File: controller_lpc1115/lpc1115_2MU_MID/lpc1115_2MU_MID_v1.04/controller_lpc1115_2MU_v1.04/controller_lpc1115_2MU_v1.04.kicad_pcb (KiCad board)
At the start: 2 copper layers, 32 x 58.1 mm, 66 parts, among them IC1 LPC1115, J1 Conn_App, J2 Conn_UI, J3 Conn_JTAG, Q1 BCP51, Q2 BC847, Q3 BC856, SW1 SW_Omron_B3FS, U1 MCP16331CH, X1 50MHz

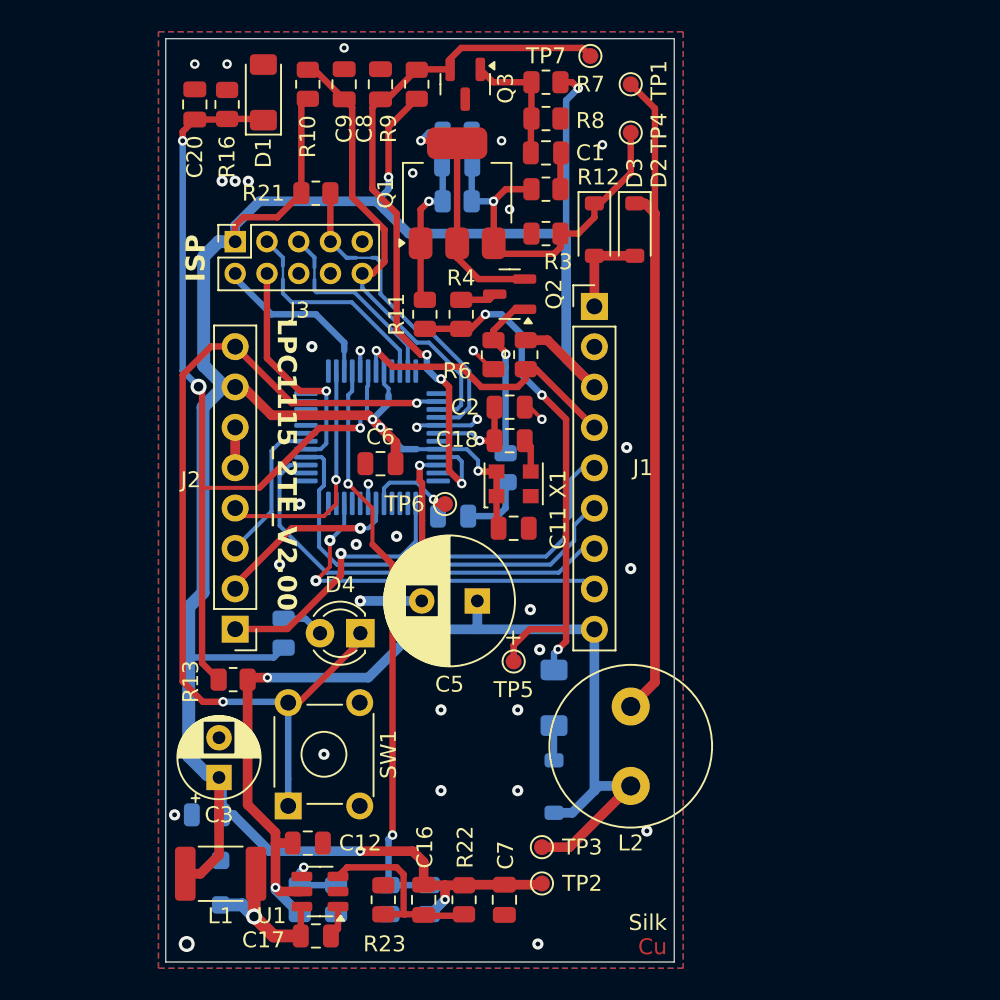
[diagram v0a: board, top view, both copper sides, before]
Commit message: update
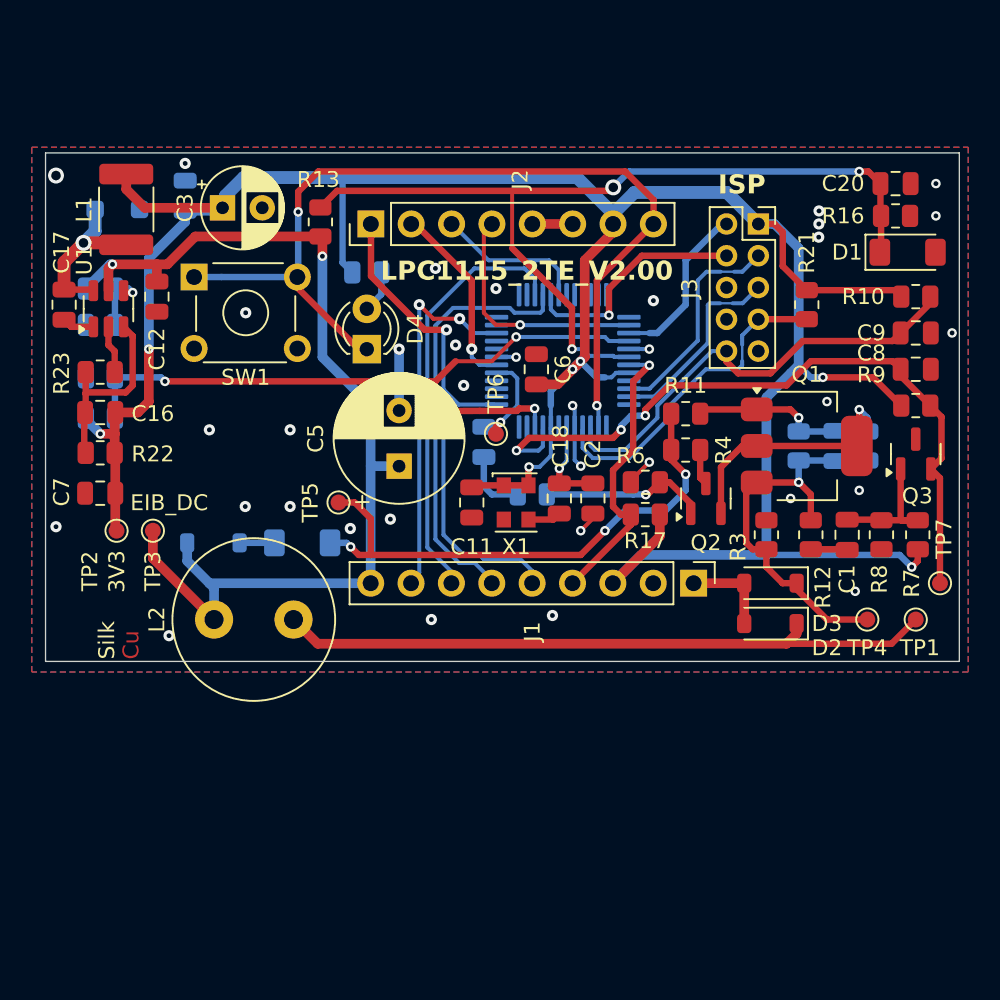
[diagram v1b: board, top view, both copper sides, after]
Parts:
- moved C20 44.4 mm to (178.5, 86.3), turned to 180 degrees
- moved D5 42.9 mm to (129.5, 87.9), turned to 0 degrees
- moved C17 42.8 mm to (126.1, 93.9), turned to 90 degrees
- moved R16 42.6 mm to (178.5, 88.3), turned to 0 degrees
- moved L1 42.2 mm to (130.1, 87.9), turned to 90 degrees
- moved D1 41.8 mm to (179.2, 90.6), turned to 0 degrees
- moved R10 40.5 mm to (179.7, 93.4), turned to 180 degrees
- moved R2 40.4 mm to (128.4, 92.9), turned to 0 degrees
- moved TP7 39.8 mm to (181.3, 111.4), turned to -90 degrees
- moved C9 39.2 mm to (179.7, 95.7), turned to 180 degrees
- moved R1 39.1 mm to (128.4, 95.2), turned to 180 degrees
- moved U1 39.0 mm to (128.9, 94.1), turned to 90 degrees
- moved C15 39.0 mm to (133.8, 87.0), turned to -90 degrees
- moved TP1 38.2 mm to (179.7, 113.7), turned to -90 degrees
- moved C8 38.2 mm to (179.7, 97.9), turned to 180 degrees
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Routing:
- net GND: track 16.0 -> 19.0 mm
- net Net-(Q3-B): track 8.01 -> 8.75 mm
- net +3V3: track 178.6 -> 177.9 mm
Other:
- board size 32 x 58.1 mm -> 57.5 x 32 mm
- board text added: "3V3"
- board text added: "<- upper side of rail mount enclosure HV side of application pcb"
- board text added: "EIB + input terminals ->"
- board text added: "EIB_DC"
